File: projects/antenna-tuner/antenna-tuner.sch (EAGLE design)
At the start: 32 parts, among them J1 Power Jack, J2 RJ45, J3 RJ45, M1 SERVO, Q1 IRF5305, Q2 BC337, U1 Arduino Pro Mini

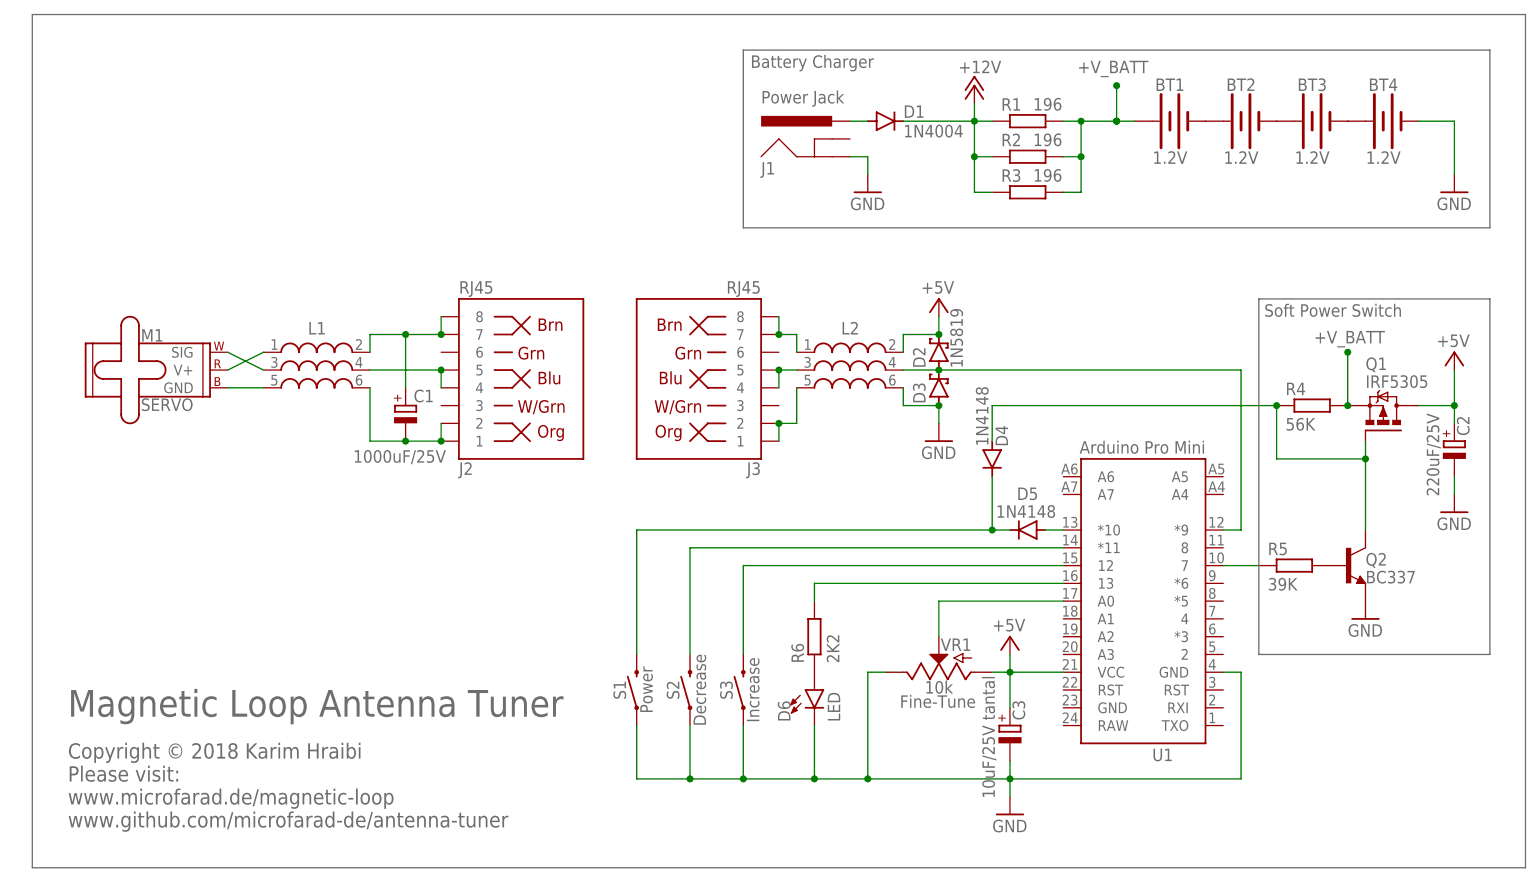
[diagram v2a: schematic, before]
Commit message: Update antenna-tuner.sch
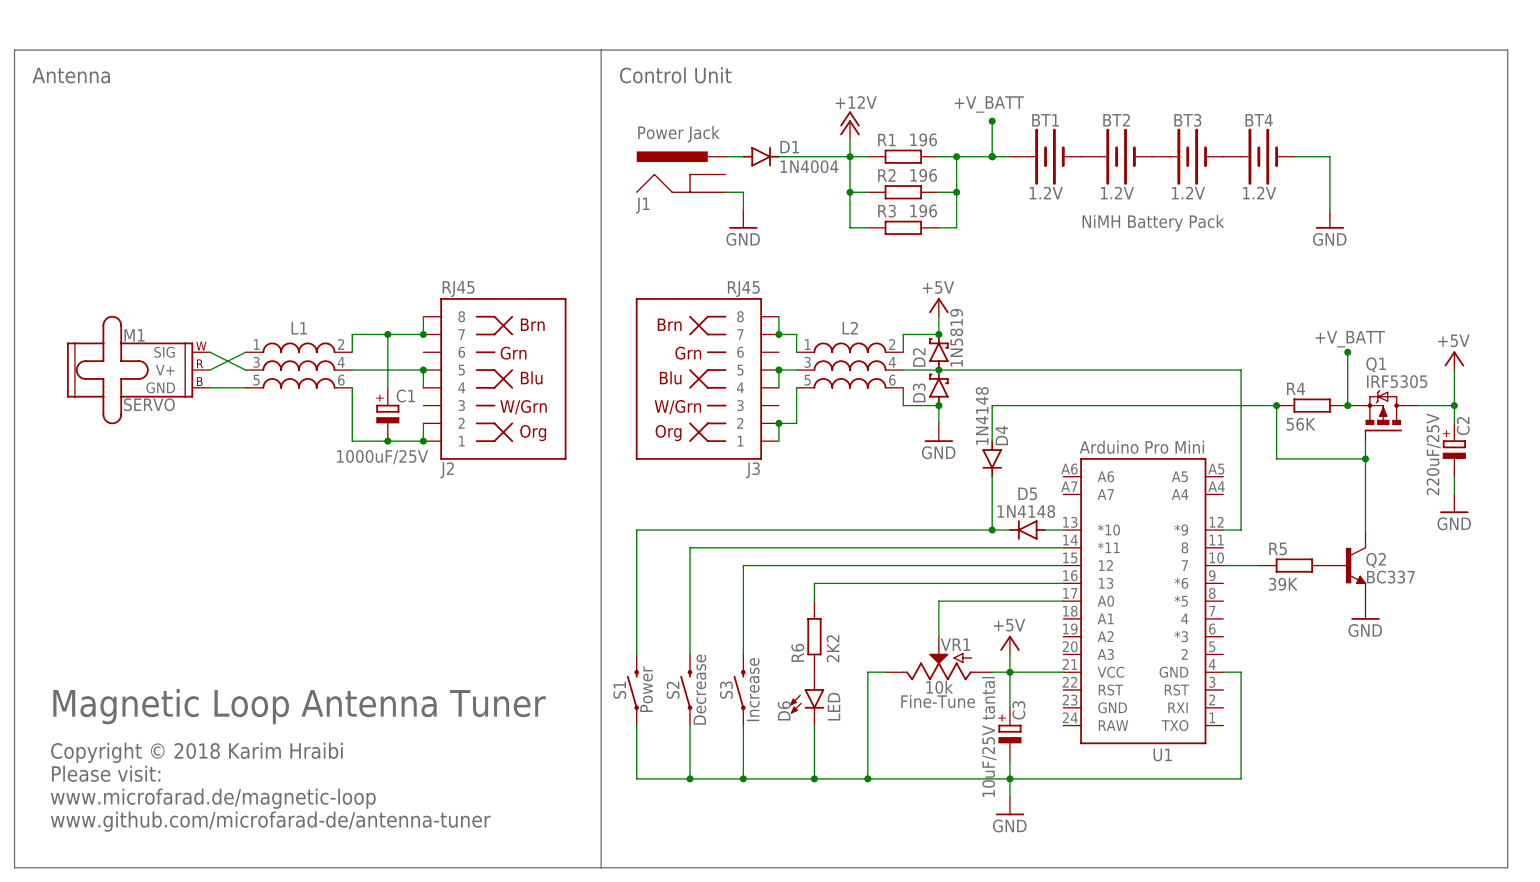
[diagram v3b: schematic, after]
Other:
- note added: "Antenna"
- note added: "Control Unit"
- note added: "NiMH Battery Pack"
- note removed: "Battery Charger"
- note removed: "Soft Power Switch"
- moved on the sheet: BT1, BT2, BT3, BT4, C1, D1, J1, J2, L1, M1, R1, R2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
